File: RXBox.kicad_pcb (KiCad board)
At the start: 4 copper layers, 60 x 16.9 mm, 76 parts, among them J1 SMA, J2 USB_A, U1 RTL2832U, U2 M24C02-WMN, U3 R820T2, U4 AP2112K-3.3, U5 74AUP1G74, U6 74LVC1G17, U7 USBLC6-2SC6, X1 19.2 MHz

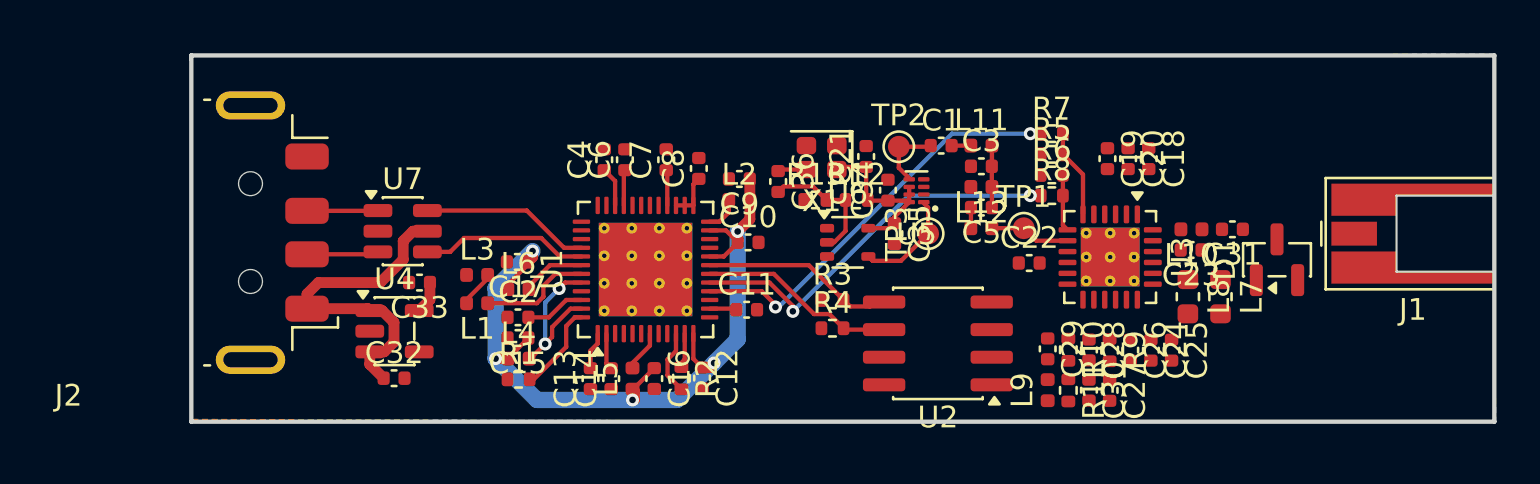
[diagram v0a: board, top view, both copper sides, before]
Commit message: done?
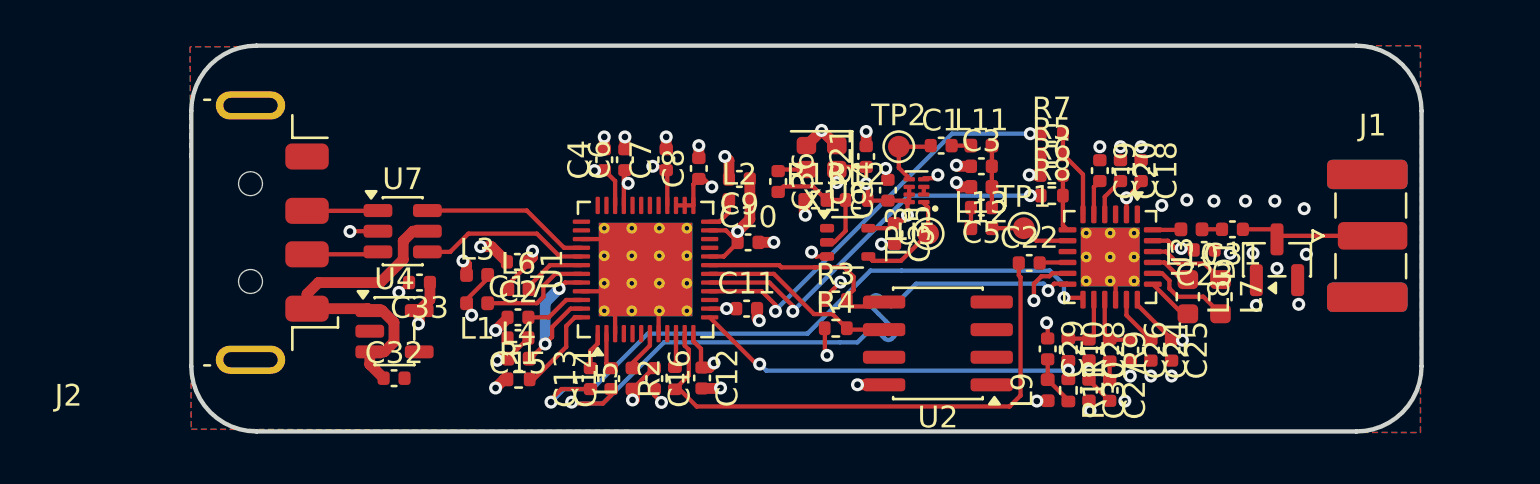
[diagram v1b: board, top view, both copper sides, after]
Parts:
- J1: footprint Connector_Coaxial:MMCX_Molex_73415-0961_Horizontal_1.0mm-PCB -> Connector_Coaxial:SMA_Samtec_SMA-J-P-H-ST-EM1_EdgeMount
- moved J1 1.85 mm to (164.9, 70.2), turned to 0 degrees
- moved C18 0.65 mm to (154.2, 67.2)
- moved C19 0.65 mm to (152.3, 67.2)
- moved C20 0.65 mm to (153.3, 67.2)
- moved C23 0.60 mm to (157.2, 70.8)
- moved R2 0.30 mm to (132.8, 76.7), turned to 90 degrees
- moved R3 0.15 mm to (140.2, 73.1)
- moved R4 0.15 mm to (140.2, 74.4)
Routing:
- net Earth: track 0.00 -> 37.0 mm, vias 0 -> 44
- net /IF_N: track 0.00 -> 31.1 mm, vias 0 -> 2
- net /IF_P: track 0.00 -> 30.0 mm, vias 0 -> 2
- net /RTL_CLK: track 1.64 -> 25.5 mm
- net /RTL_IF_AGC: track 0.00 -> 18.4 mm, vias 0 -> 2
- net +3V3: track 9.59 -> 27.4 mm, vias 0 -> 15
- net +1V2: track 41.9 -> 53.9 mm, vias 5 -> 7
- net Net-(J1-In): track 0.00 -> 6.50 mm
- net Net-(U3-TF2P): track 0.00 -> 4.10 mm
- net Net-(U3-TF1P): track 0.00 -> 3.65 mm
- net /IF_AGC: track 0.00 -> 2.89 mm
- net Net-(U3-CP): track 0.00 -> 2.87 mm
- net /RTL_3V3: track 6.71 -> 9.21 mm, vias 0 -> 4
- net Net-(C29-Pad2): track 0.00 -> 2.33 mm
- net Net-(U3-VDD_PLL): track 0.00 -> 2.31 mm
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- added copper zone on In2.Cu, net +3V3
- added copper zone on In2.Cu, net /RTL_3V3
- removed copper zone on In2.Cu, net Earth
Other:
- board size 60 x 16.9 mm -> 56.6 x 17.8 mm
